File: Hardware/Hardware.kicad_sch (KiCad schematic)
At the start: 40 parts, among them J1 USB4105-GF-A, J2 Conn_01x06_Socket, J3 Conn_01x06_Socket, SW1 SW_Push, SW2 SW_Push, U1 ESP32-C3-MINI-1-N4, U3 LM1117MP-3.3

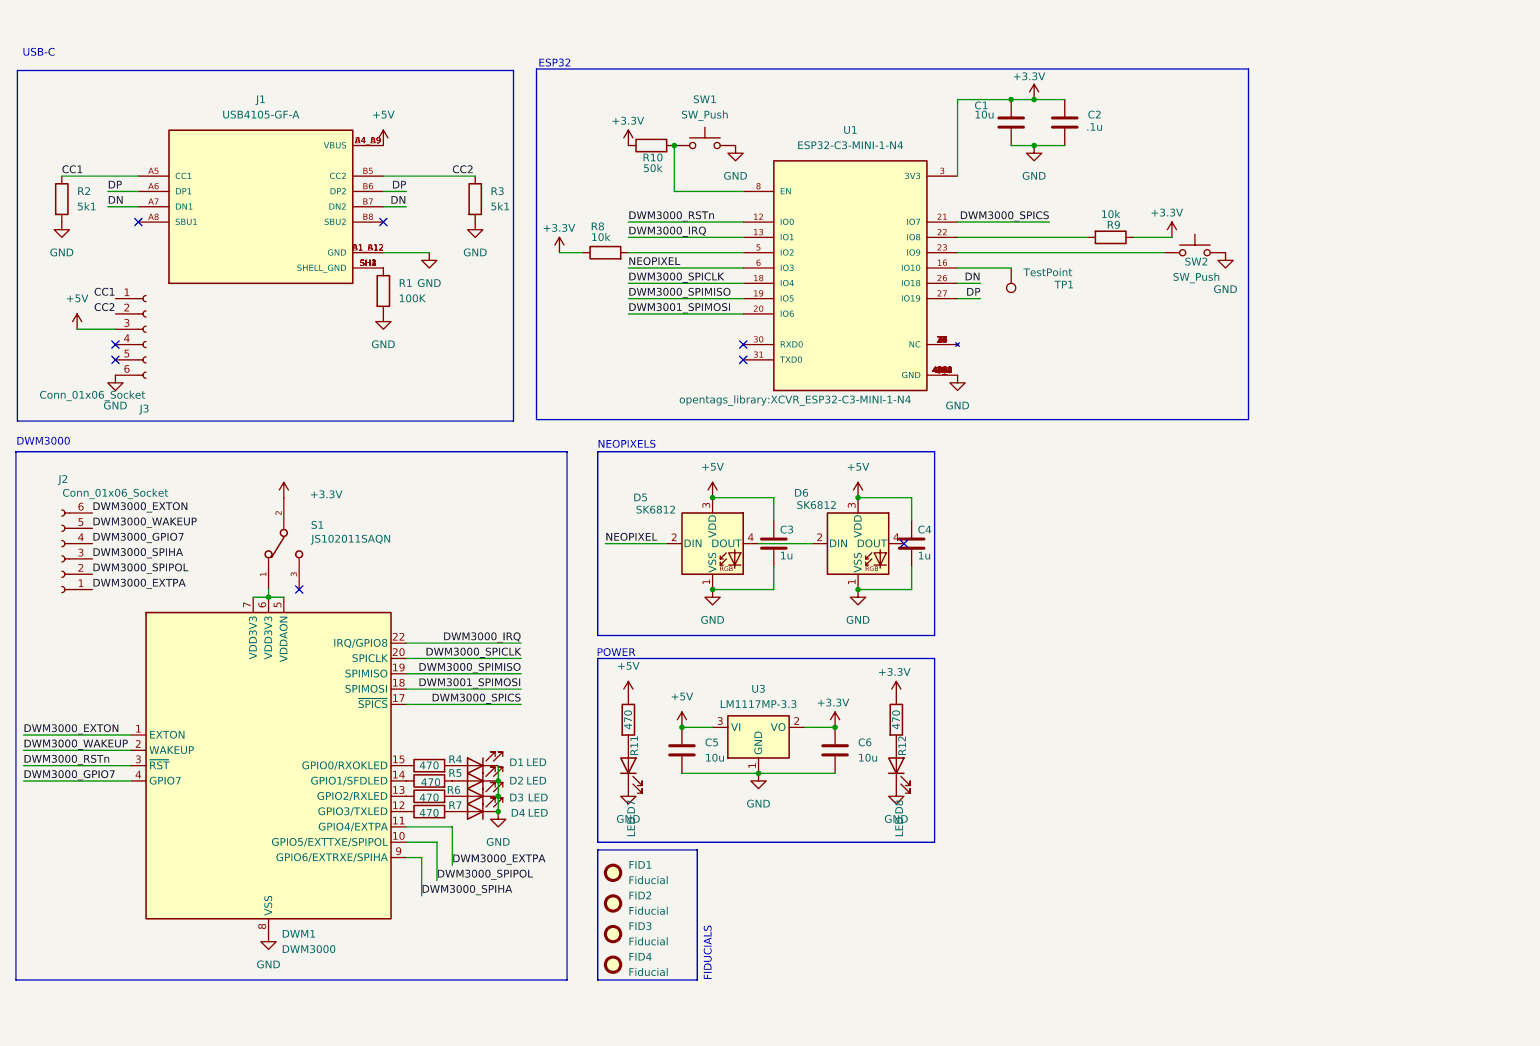
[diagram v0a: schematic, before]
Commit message: hardware updates
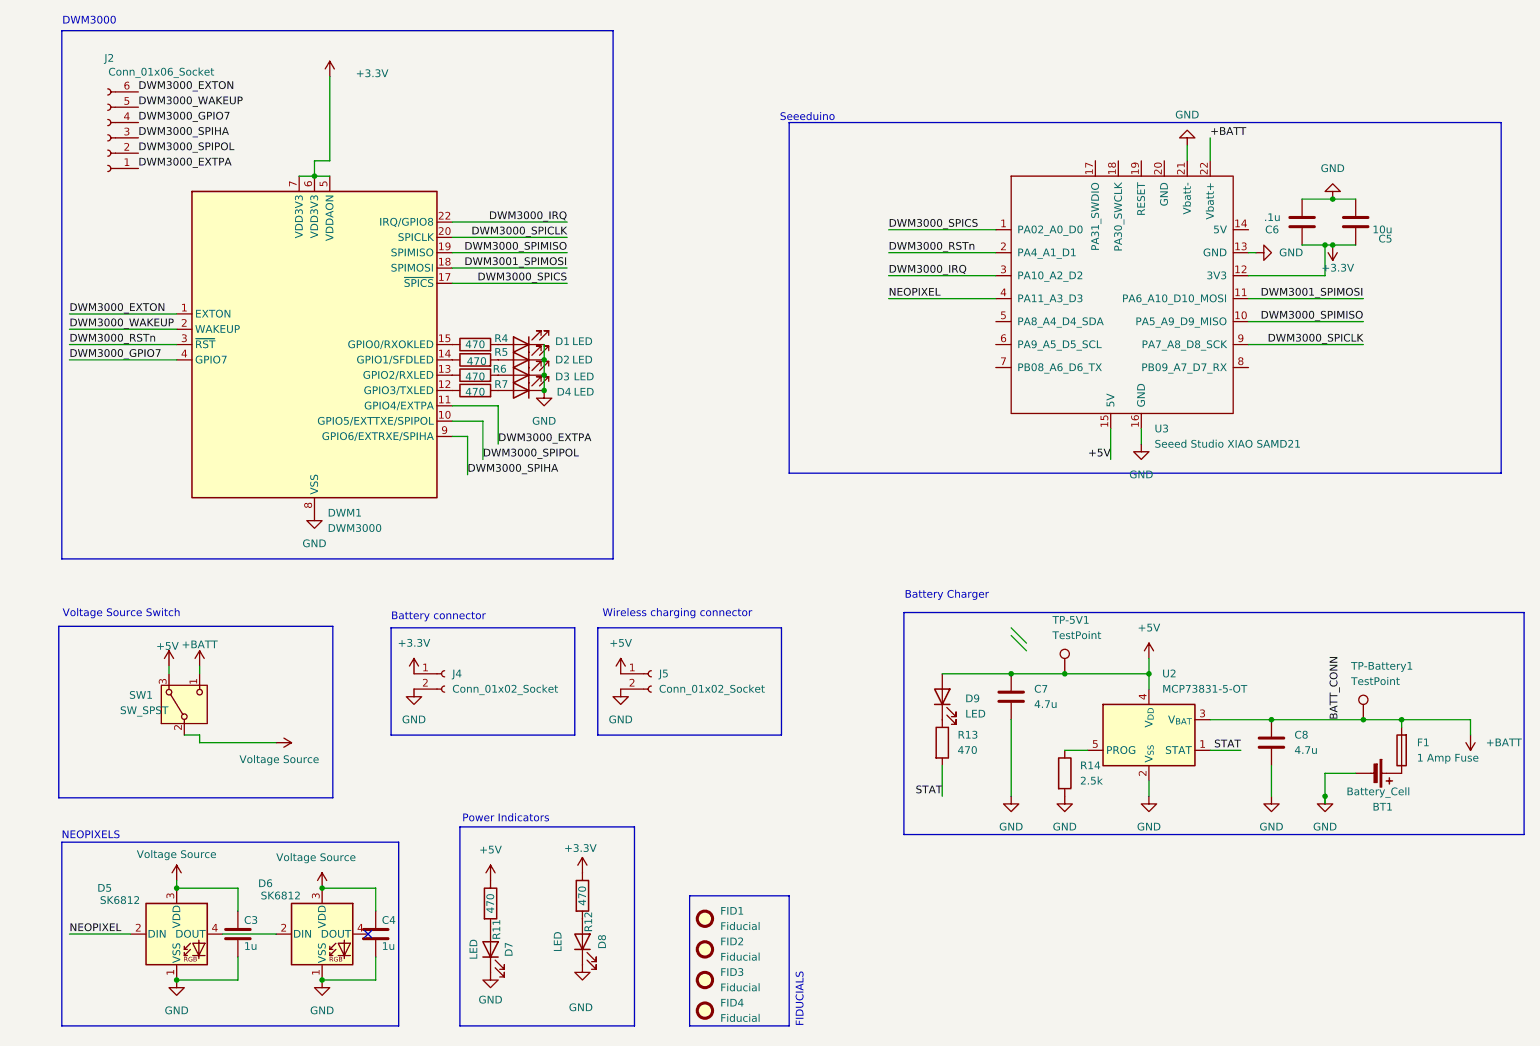
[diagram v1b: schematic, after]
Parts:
- removed C1: 10u, Capacitor_SMD:C_0603_1608Metric, symbol Device:C
- removed C2: .1u, Capacitor_SMD:C_0603_1608Metric, symbol Device:C
- removed J1: USB4105-GF-A, opentags_library:GCT_USB4105-GF-A, symbol opentags_library:USB4105-GF-A
- removed J3: Conn_01x06_Socket, Connector_PinHeader_1.00mm:PinHeader_1x06_P1.00mm_Vertical, symbol Connector:Conn_01x06_Socket
- removed R1: 100K, Resistor_SMD:R_0603_1608Metric, symbol Device:R
- removed R10: 50k, Resistor_SMD:R_0603_1608Metric, symbol Device:R
- removed R2, R3: 5k1, Resistor_SMD:R_0603_1608Metric, symbol Device:R
- removed R8, R9: 10k, Resistor_SMD:R_0603_1608Metric, symbol Device:R
- removed S1: JS102011SAQN, opentags_library:SW_JS102011SAQN, symbol opentags_library:JS102011SAQN
- removed SW1, SW2: SW_Push, Button_Switch_SMD:SW_SPST_PTS810, symbol Switch:SW_Push
- removed TP1: TestPoint, TestPoint:TestPoint_Pad_D2.0mm, symbol Connector:TestPoint
- removed U1: ESP32-C3-MINI-1-N4, opentags_library:XCVR_ESP32-C3-MINI-1-N4, symbol opentags_library:ESP32-C3-MINI-1-N4
- removed U3: LM1117MP-3.3, Package_TO_SOT_SMD:SOT-223-3_TabPin2, symbol Regulator_Linear:LM1117MP-3.3
- added BT1: Battery_Cell, Connector_PinHeader_2.54mm:PinHeader_1x02_P2.54mm_Vertical, symbol Device:Battery_Cell
- added C7, C8: 4.7u, Capacitor_SMD:C_0603_1608Metric, symbol Device:C
- added D9: LED, Resistor_SMD:R_0603_1608Metric, symbol Device:LED
- added F1: 1 Amp Fuse, Fuse:Fuse_0603_1608Metric, symbol Device:Fuse
- added J4, J5: Conn_01x02_Socket, Connector_PinHeader_2.54mm:PinHeader_1x02_P2.54mm_Vertical, symbol Connector:Conn_01x02_Socket
- added R13: 470, Resistor_SMD:R_0603_1608Metric, symbol Device:R
- added R14: 2.5k, Resistor_SMD:R_0603_1608Metric, symbol Device:R
- added SW1: SW_SPST, opentags_library:SW_JS102011SAQN, symbol Switch:SW_SPDT_321
- added TP-5V1, TP-Battery1: TestPoint, TestPoint:TestPoint_Pad_D2.0mm, symbol Connector:TestPoint
- added U2: MCP73831-5-OT, Package_TO_SOT_SMD:SOT-23-5, symbol Battery_Management:MCP73831-5-OT
- added U3: Seeed Studio XIAO SAMD21, Seeed Studio XIAO Series Library:XIAO-nRF52840-Sense-14P-2.54-21X17.8MM, symbol Seeed_Studio_XIAO_Series:Seeed Studio XIAO SAMD21
- C6: value 10u -> .1u
- J2: footprint Connector_PinHeader_1.00mm:PinHeader_1x06_P1.00mm_Vertical -> Connector_PinHeader_2.00mm:PinHeader_1x06_P2.00mm_Vertical
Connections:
- net +3.3V: now also C5.1, DWM1.5 (VDDAON), DWM1.6 (VDD3V3), DWM1.7 (VDD3V3), J4.1 (Pin_1), U3.12 (3V3)
- net +5V: now also C7.1, D9.2 (A), J5.1 (Pin_1), SW1.3 (A), TP-5V1.1, U2.4 (V_{DD}), U3.15 (5V); no longer C3.2, C4.2, C5.1, D5.3 (VDD), D6.3 (VDD)
- net DWM3000_IRQ: now also U3.3 (PA10_A2_D2)
- net DWM3000_RSTn: now also U3.2 (PA4_A1_D1)
- net DWM3000_SPICLK: now also U3.9 (PA7_A8_D8_SCK)
- net DWM3000_SPICS: now also U3.1 (PA02_A0_D0)
- net DWM3000_SPIMISO: now also U3.10 (PA5_A9_D9_MISO)
- net DWM3001_SPIMOSI: now also U3.11 (PA6_A10_D10_MOSI)
- net GND: now also BT1.2 (-), C7.2, C8.2, J4.2 (Pin_2), J5.2 (Pin_2), R14.2, U2.2 (V_{SS}), U3.13 (GND), U3.16 (GND), U3.21 (Vbatt-)
- net NEOPIXEL: now also U3.4 (PA11_A3_D3)
- new net: R14.1, U2.5 (PROG)
- new net: BT1.1 (+), F1.1
- new net: D9.1 (K), R13.1
- new net +BATT: C8.1, F1.2, SW1.1 (C), TP-Battery1.1, U2.3 (V_{BAT}), U3.22 (Vbatt+)
- new net STAT: R13.2, U2.1 (STAT)
- new net Voltage Source: C3.2, C4.2, D5.3 (VDD), D6.3 (VDD), SW1.2 (B)
- no-connect marks 8 -> 1
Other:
- note added: "Battery Charger"
- note added: "Battery connector"
- note added: "Power Indicators"
- note added: "Seeeduino"
- note added: "Voltage Source Switch"
- note added: "Wireless charging connector"
- note removed: "ESP32"
- note removed: "POWER"
- note removed: "USB-C"
- moved on the sheet: C3, C4, D1, D2, D3, D4, D5, D6, D7, D8, DWM1, FID1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
